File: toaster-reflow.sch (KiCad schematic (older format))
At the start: 19 parts, among them J1 1935161, J2 1935161, J3 Raspberry_Pi_2_3, J4 Conn_01x04, J6 Conn_01x03, K1 1-1415899-3, Q1 Q_NMOS_GSD, Q2 Q_NMOS_GSD, U1 3.3V Ref

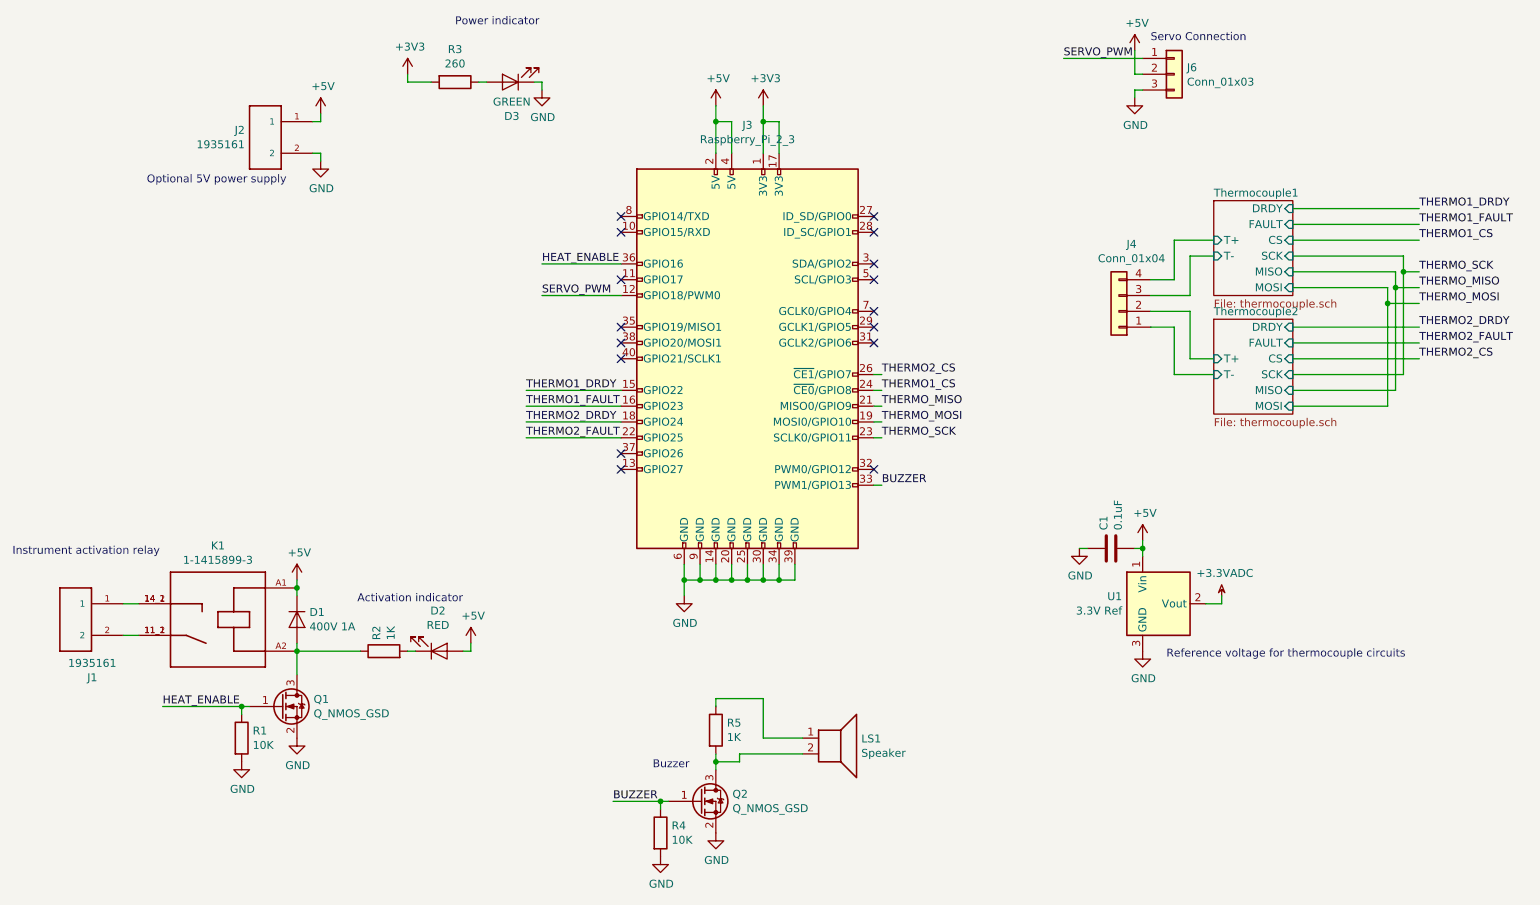
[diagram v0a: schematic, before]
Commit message: update some stuff
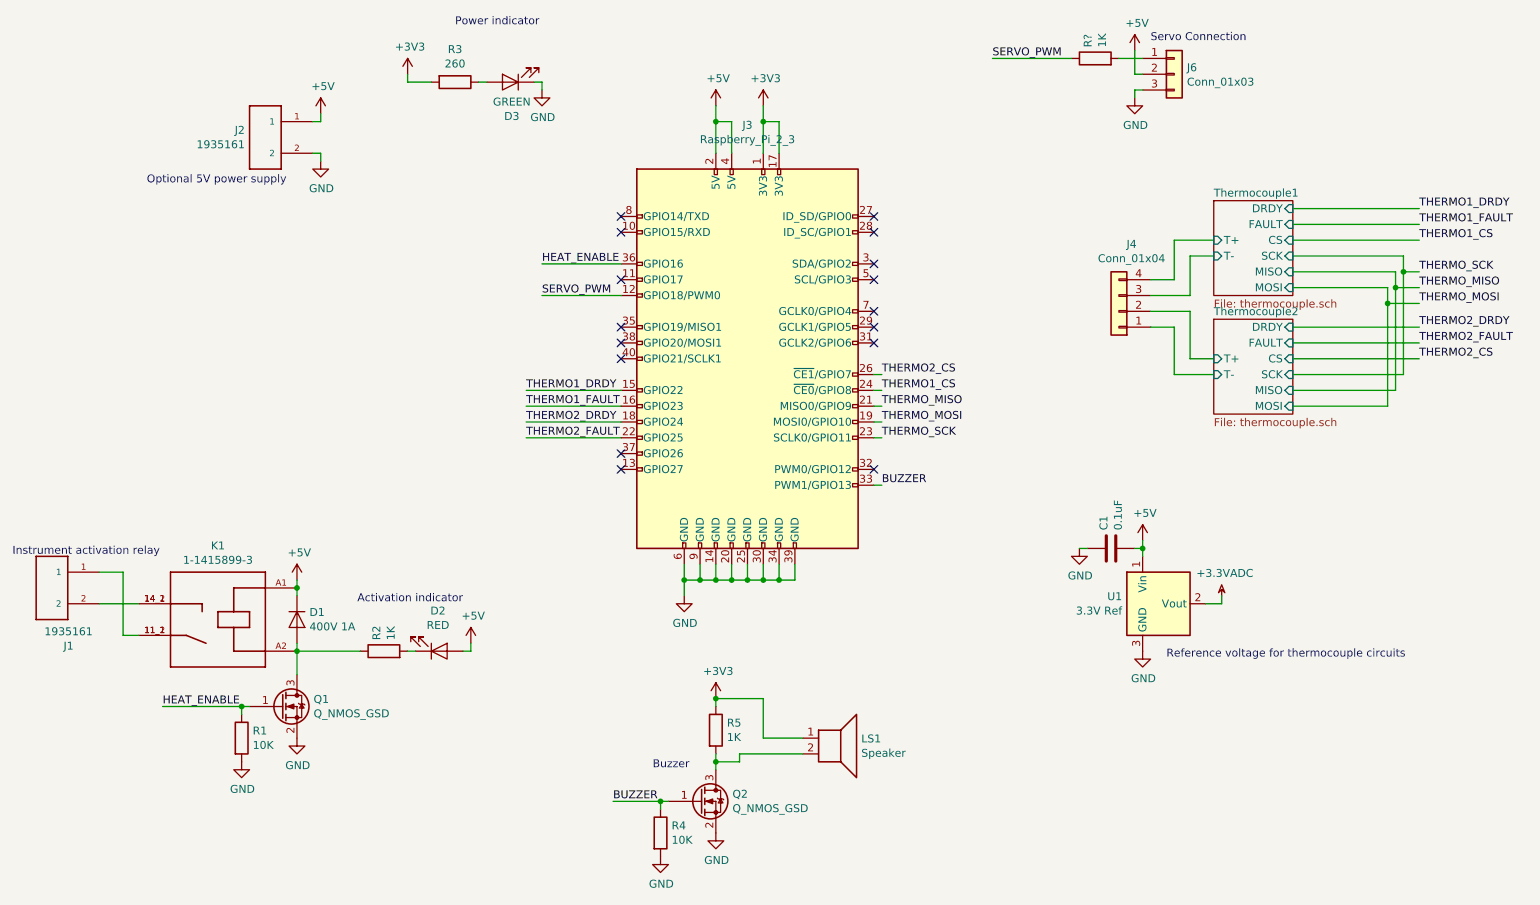
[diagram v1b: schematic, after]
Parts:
- added R?: 1K, Resistor_SMD:R_0603_1608Metric, symbol Device:R
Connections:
- net +3V3: now also LS1.1, R5.1
- net SERVO_PWM: now also R?.1; no longer J6.1 (Pin_1)
- net at K1.11_1 (11), K1.11_2 (11): now also J1.1; no longer J1.2
- net at K1.14_1 (14), K1.14_2 (14): now also J1.2; no longer J1.1
- new net: J6.1 (Pin_1), R?.2
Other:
- moved on the sheet: J1
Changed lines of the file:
@@
 $EndComp
-Wire Wire Line
-	1550 5650 1650 5650
 Wire Wire Line
 	1550 5850 1650 5850
@@
 L 1935161:1935161 J1
 U 1 1 5B8AC1A4
-P 1250 5750
-F 0 "J1" H 1145 5383 50  0000 C CNN
-F 1 "1935161" H 1145 5474 50  0000 C CNN
-F 2 "1935161:PHOENIX_1935161" H 1250 5750 50  0001 L BNN
-F 3 "Phoenix Contact" H 1250 5750 50  0001 L BNN
-F 4 "277-1667-ND" H 1250 5750 50  0001 C CNN "DigikeyPartNumber"
-F 5 "None" H 1250 5750 50  0001 L BNN "Field4"
-F 6 "Conn Terminal Blocks 2 POS 5mm Solder ST Thru-Hole 16A" H 1250 5750 50  0001 L BNN "Field5"
-F 7 "None" H 1250 5750 50  0001 L BNN "Field6"
-F 8 "1935161" H 1250 5750 50  0001 L BNN "Field7"
-F 9 "Unavailable" H 1250 5750 50  0001 L BNN "Field8"
-	1    1250 5750
+P 1100 5550
+F 0 "J1" H 995 5183 50  0000 C CNN
+F 1 "1935161" H 995 5274 50  0000 C CNN
+F 2 "1935161:PHOENIX_1935161" H 1100 5550 50  0001 L BNN
+F 3 "Phoenix Contact" H 1100 5550 50  0001 L BNN
+F 4 "277-1667-ND" H 1100 5550 50  0001 C CNN "DigikeyPartNumber"
+F 5 "None" H 1100 5550 50  0001 L BNN "Field4"
+F 6 "Conn Terminal Blocks 2 POS 5mm Solder ST Thru-Hole 16A" H 1100 5550 50  0001 L BNN "Field5"
+F 7 "None" H 1100 5550 50  0001 L BNN "Field6"
+F 8 "1935161" H 1100 5550 50  0001 L BNN "Field7"
+F 9 "Unavailable" H 1100 5550 50  0001 L BNN "Field8"
+	1    1100 5550
 	-1   0    0    -1
 $EndComp
@@
 	4700 4300 4100 4300
 Wire Wire Line
-	7500 2200 8000 2200
-Text Label 7500 2200 0    50   ~ 0
+	7050 2200 7550 2200
+Text Label 7050 2200 0    50   ~ 0
 SERVO_PWM
 $Comp
@@
 Text Notes 4900 6700 0    50   ~ 0
 Buzzer
+Wire Wire Line
+	1400 5650 1650 5650
+Wire Wire Line
+	1400 5450 1550 5450
+Wire Wire Line
+	1550 5450 1550 5850
+$Comp
+L Device:R R?
+U 1 1 5BE2B437
+P 7700 2200
+F 0 "R?" H 7770 2246 50  0000 L CNN
+F 1 "1K" H 7770 2155 50  0000 L CNN
+F 2 "Resistor_SMD:R_0603_1608Metric" V 7630 2200 50  0001 C CNN
+F 3 "https://www.rohm.com/datasheet/ESR01MZPF/esr-e" H 7700 2200 50  0001 C CNN
+F 4 "RHM1.0KDCT-ND" H 7700 2200 50  0001 C CNN "DigikeyPartNumber"
+	1    7700 2200
+	0    -1   -1   0
+$EndComp
+Wire Wire Line
+	8000 2200 7850 2200
+$Comp
+L power:+3V3 #PWR?
+U 1 1 5BE3EC4D
+P 5300 6250
+F 0 "#PWR?" H 5300 6100 50  0001 C CNN
+F 1 "+3V3" H 5315 6423 50  0000 C CNN
+F 2 "" H 5300 6250 50  0001 C CNN
+F 3 "" H 5300 6250 50  0001 C CNN
+	1    5300 6250
+	1    0    0    -1
+$EndComp
+Connection ~ 5300 6250
 $EndSCHEMATC
